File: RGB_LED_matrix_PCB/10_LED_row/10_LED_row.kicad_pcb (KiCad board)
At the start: 2 copper layers, 20 parts, among them U1 WS2815F, U10 WS2815F, U2 WS2815F, U3 WS2815F, U4 WS2815F, U5 WS2815F, U6 WS2815F, U7 WS2815F, U8 WS2815F, U9 WS2815F

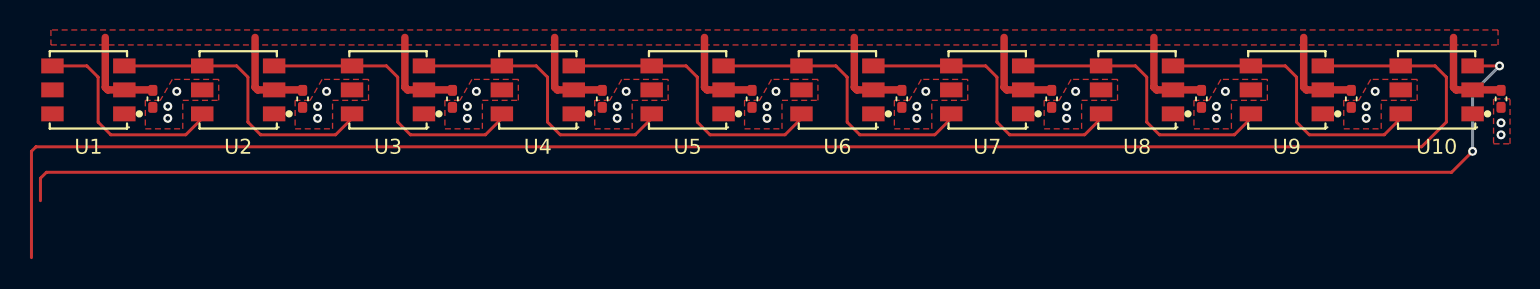
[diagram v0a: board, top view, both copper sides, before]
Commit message: Fixed some issues with the layout
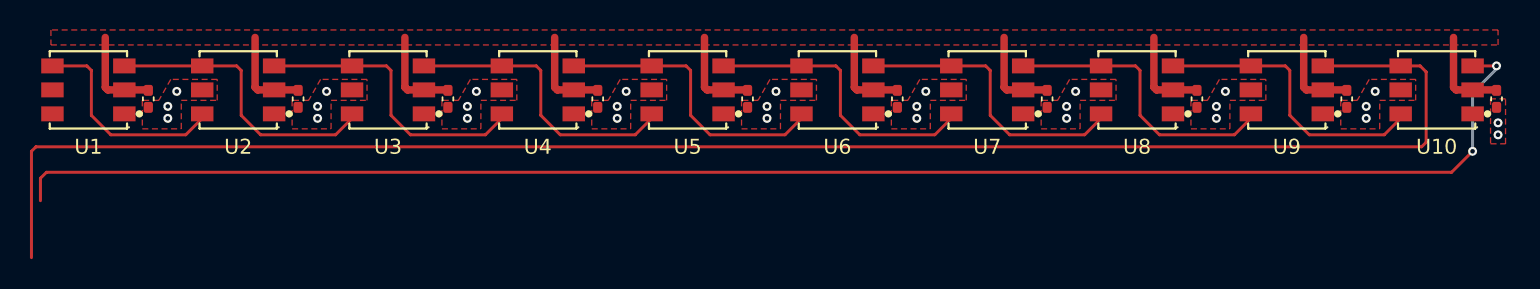
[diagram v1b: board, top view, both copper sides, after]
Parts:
- moved C10 0.30 mm to (193.0, 99.6)
- moved C4 0.30 mm to (133.0, 99.6)
- moved C5 0.30 mm to (143.0, 99.6)
- moved C6 0.30 mm to (153.0, 99.6)
- moved C7 0.30 mm to (163.0, 99.6)
- moved C8 0.30 mm to (173.0, 99.6)
- moved C9 0.30 mm to (183.0, 99.6)
- moved C1 0.30 mm to (103.0, 99.6)
- moved C2 0.30 mm to (113.0, 99.6)
- moved C3 0.30 mm to (123.0, 99.6)
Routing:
- net +12V: track 65.9 -> 62.9 mm
- net /DOUT2: track 113.9 -> 112.2 mm
